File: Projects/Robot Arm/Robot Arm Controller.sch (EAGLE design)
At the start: 48 parts, among them IC1 U_FTDICHIP_FT232RL, J1 ICSP HEADER, P1 P_USB_MINIUX60A-MB-5ST, P2 +12V INPUT, U1 UA78M05CDCY, U2 TPS71550DCKR, U3 U_ATMEGA328P-AU, U4 U_5VSWITCHER_TL2575-05IKTTR, U5 U_STEPPER_DRIVER_A4988ALT1, Y1 CSTCE16M0V13

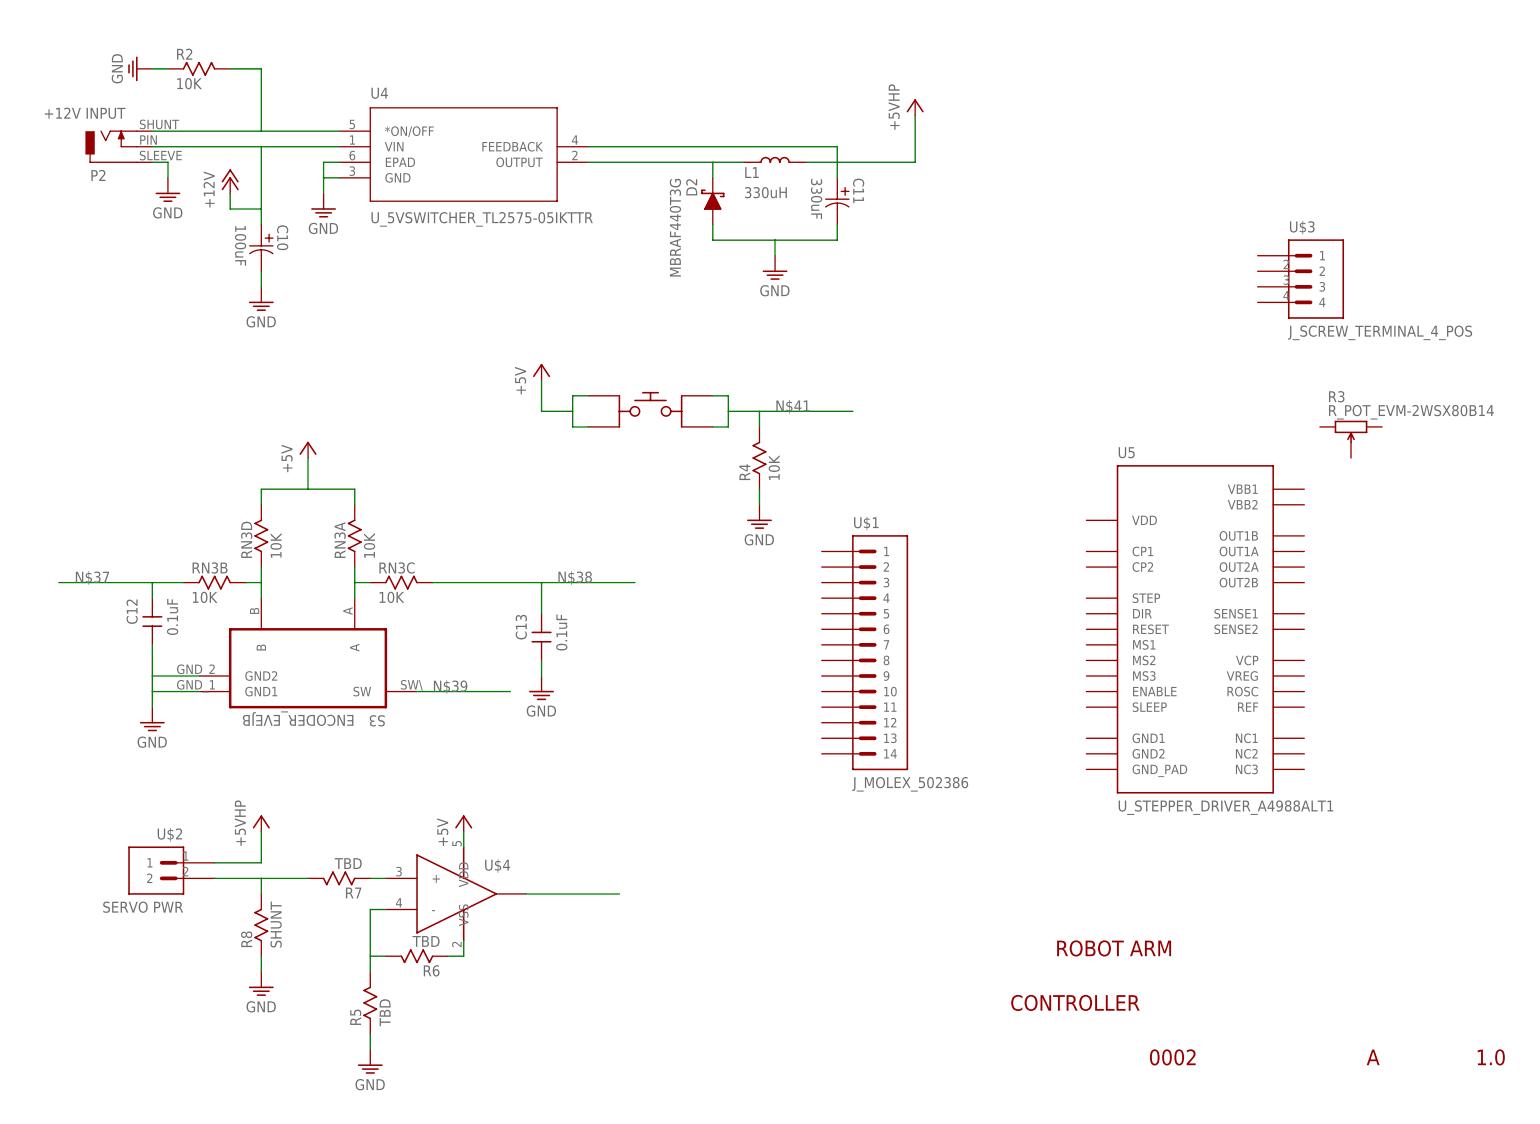
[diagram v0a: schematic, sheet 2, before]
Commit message: Full schematic up for review
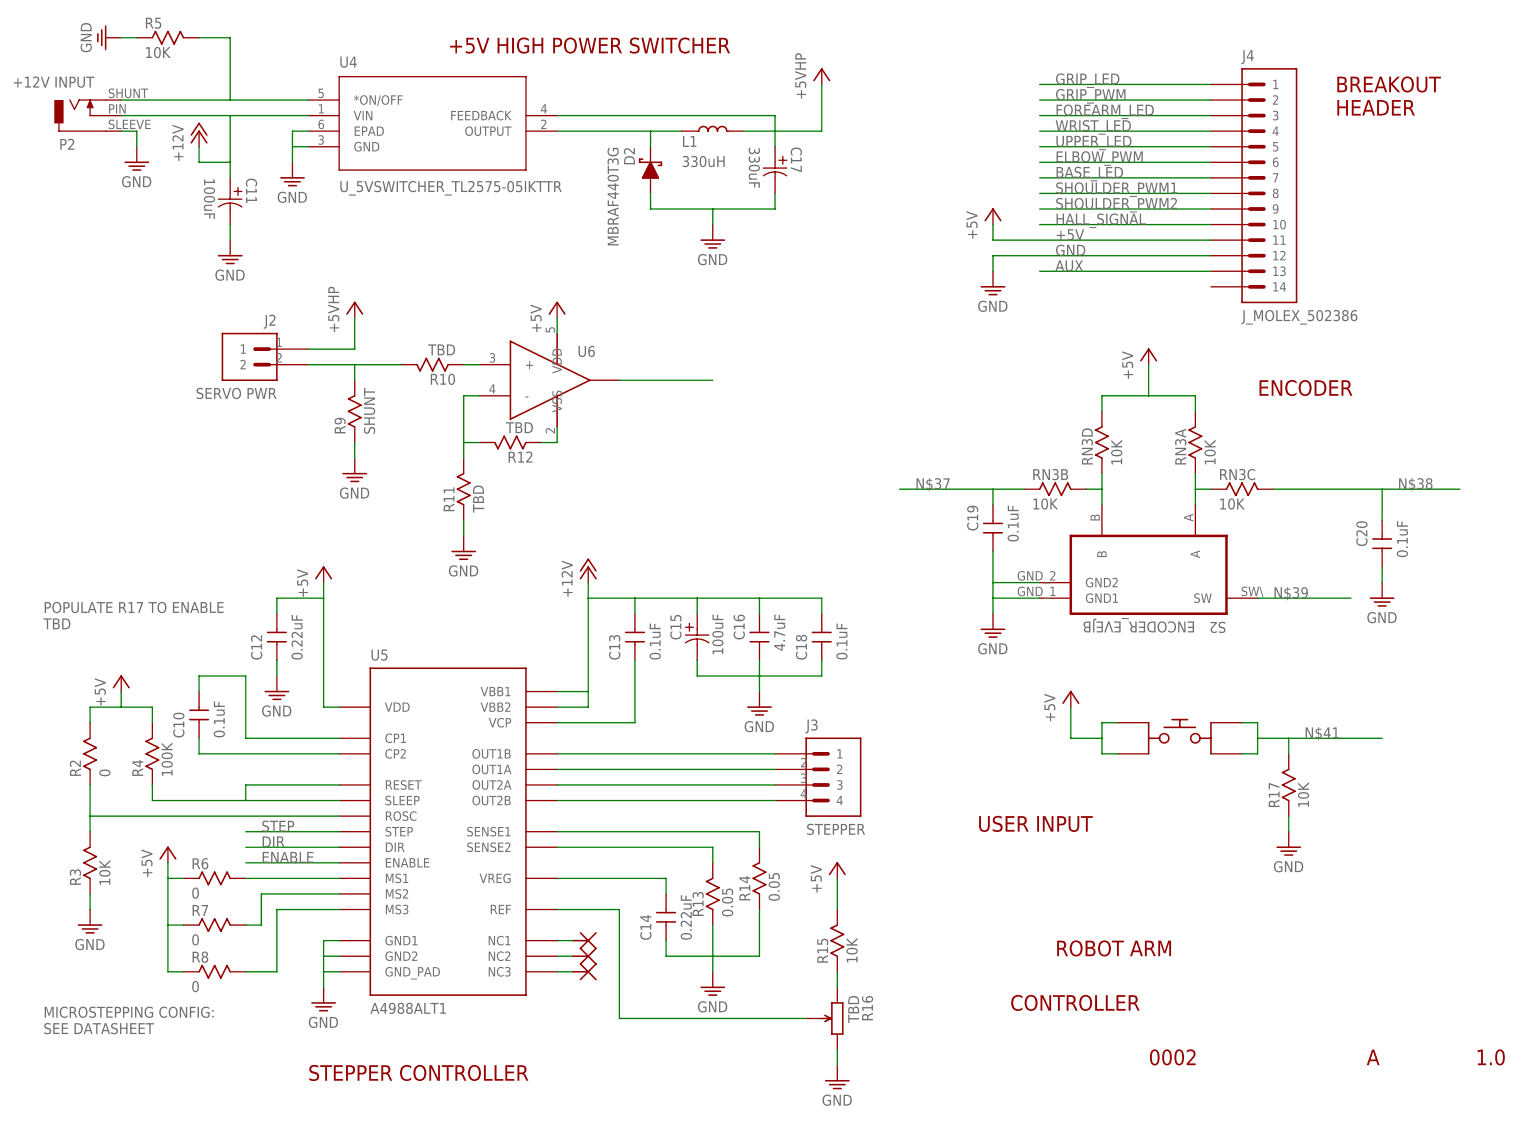
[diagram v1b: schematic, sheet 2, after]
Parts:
- removed U$1: J_MOLEX_502386, devon:J_MOLEX_502386
- removed U$2: SERVO PWR, devon:J_SCREW_TERMINAL_2_POS
- removed U$3: J_SCREW_TERMINAL_4_POS, devon:J_SCREW_TERMINAL_4_POS
- removed U$4: U_OPAMP_MCP6001T-E/OT, devon:U_OPAMP_MCP6001T-E/OT
- added C14: 0.22uF, devon:C_CAPACITORC0805
- added C15: 100uF, devon:C_CAPACITOR_ALUMINUM_PCAP_SVP_F12
- added C16: 4.7uF, devon:C_CAPACITORC1206
- added C17: 330uF, devon:C_CAPACITOR_ALUMINUM_PCAP_SVP_F12
- added C18, C19, C20: 0.1uF, devon:C_CAPACITORC0805
- added J2: SERVO PWR, devon:J_SCREW_TERMINAL_2_POS
- added J3: STEPPER, devon:J_SCREW_TERMINAL_4_POS
- added J4: J_MOLEX_502386, devon:J_MOLEX_502386
- added R10, R11, R12: TBD, devon:R_RESISTOR0805
- added R13, R14: 0.05, devon:R_RESISTOR1206
- added R15, R17: 10K, devon:R_RESISTOR0805
- added R16: TBD, devon:R_POT_EVM-2WSX80B14
- added R9: SHUNT, devon:R_RESISTOR1206
- added U6: U_OPAMP_MCP6001T-E/OT, devon:U_OPAMP_MCP6001T-E/OT
- C10: value 100uF -> 0.1uF; device devon:C_CAPACITOR_ALUMINUM_PCAP_SVP_F12 -> devon:C_CAPACITORC0805
- C11: value 330uF -> 100uF
- C12: value 0.1uF -> 0.22uF
- R2: value 10K -> 0
- R3: value R_POT_EVM-2WSX80B14 -> 10K; device devon:R_POT_EVM-2WSX80B14 -> devon:R_RESISTOR0805
- R4: value 10K -> 100K
- R5: value TBD -> 10K
- R6, R7: value TBD -> 0
- R8: value SHUNT -> 0; device devon:R_RESISTOR1206 -> devon:R_RESISTOR0805
- S2: value S_BUTTON_TACTILE_PTS645 -> ENCODER_EVEJB; device devon:S_BUTTON_TACTILE_PTS645 -> devon:S_ENCODER_EVEJB
- S3: value ENCODER_EVEJB -> S_BUTTON_TACTILE_PTS645; device devon:S_ENCODER_EVEJB -> devon:S_BUTTON_TACTILE_PTS645
- U5: value U_STEPPER_DRIVER_A4988ALT1 -> A4988ALT1
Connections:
- new net AUX: J4.13
- new net BASE_LED: J4.7
- new net DIR: U5.DIR
- new net ELBOW_PWM: J4.6
- new net ENABLE: U5.ENABLE
- new net FOREARM_LED: J4.3
- new net GRIP_LED: J4.1
- new net GRIP_PWM: J4.2
- new net HALL_SIGNAL: J4.10
- new net N$40: J3.1, U5.OUT1B
- new net N$46: J3.2, U5.OUT1A
- new net N$47: J3.3, U5.OUT2A
- new net N$48: J3.4, U5.OUT2B
- new net N$50: C14.1, U5.VREG
- new net N$51: R13.2, U5.SENSE2
- new net N$52: R15.1, R16.1
- new net N$53: R14.2, U5.SENSE1
- new net N$54: R16.2, U5.REF
- new net N$55: U5.NC1
- new net N$56: U5.NC2
- new net N$57: U5.NC3
- new net N$58: C13.2, U5.VCP
- new net N$59: C10.2, U5.CP2
- new net N$60: C10.1, U5.CP1
- new net N$61: R7.2, U5.MS2
- new net N$62: R6.2, U5.MS1
- new net N$63: R8.2, U5.MS3
- new net N$64: R4.1, U5.RESET, U5.SLEEP
- new net N$65: R2.1, R3.2, U5.ROSC
- new net SHOULDER_PWM1: J4.8
- new net SHOULDER_PWM2: J4.9
- new net STEP: U5.STEP
- new net UPPER_LED: J4.5
- new net WRIST_LED: J4.4
- net +12V: now also C11.11, C13.1, C15.11, C16.2, C18.1, U5.VBB1, U5.VBB2; no longer C10.11
- net +5V: now also C12.1, C17.11, J2.1, J4.11, R15.2, R2.2, R4.2, R6.1, R7.1, R8.1, S3.1, S3.2, U5.VDD, U6.VDD; no longer C11.11, S2.1, S2.2, U$2.1, U$4.VDD
- net GND: now also C12.2, C14.2, C15.22, C16.1, C17.22, C18.2, C19.1, C20.1, J4.12, R11.1, R13.1, R14.1, R16.3, R17.1, R3.1, R9.1, S2.GND1, S2.GND2, U5.GND1, U5.GND2, U5.GND_PAD; no longer C10.22, C12.1, R2.1, R4.1, R8.1, S3.GND1, S3.GND2
- net N$34: now also S2.B; no longer S3.B
- net N$35: now also R5.2; no longer R2.2
- net N$36: now also S2.A; no longer S3.A
- net N$37: now also C19.2; no longer C12.2
- net N$38: now also C20.2; no longer C13.2
- net N$39: now also S2.SW; no longer S3.SW
- net N$41: now also R17.2, S3.3, S3.4; no longer R4.2, S2.3, S2.4
- net N$42: now also R12.1, U6.VSS; no longer R6.1, U$4.VSS
- net N$43: now also R10.1, U6.+; no longer R7.1, U$4.+
- net N$44: now also R11.2, R12.2, U6.-; no longer R5.2, R6.2, U$4.-
- net N$45: now also J2.2, R10.2, R9.2; no longer R7.2, R8.2, U$2.2
- net N$49: now also U6.VOUT; no longer U$4.VOUT
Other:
- note added: "+5V HIGH POWER SWITCHER"
- note added: "BREAKOUT HEADER"
- note added: "ENCODER"
- note added: "MICROSTEPPING CONFIG: SEE DATASHEET"
- note added: "POPULATE R17 TO ENABLE TBD"
- note added: "STEPPER CONTROLLER"
- note added: "USER INPUT"
- moved on the sheet: C11, C12, C13, D2, L1, P2, R2, R4, R5, R6, R7, R8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
